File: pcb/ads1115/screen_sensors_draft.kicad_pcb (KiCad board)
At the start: 2 copper layers, 42 x 32 mm, 16 parts, among them J1 WAVESHARE_I2C, J2 BOILER_PROBE, J3 XDB401_ANALOG, U1 ADS1115IDGSR, U2 SHT40-AD1B

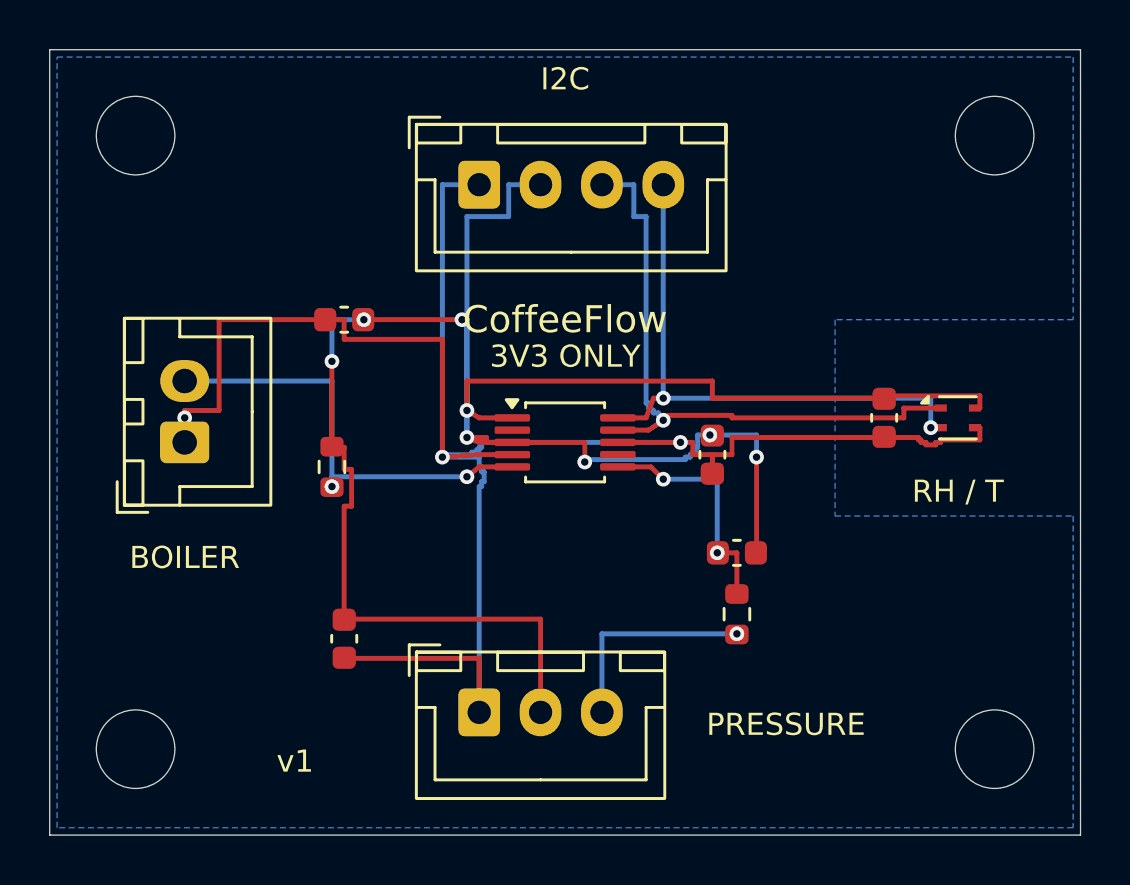
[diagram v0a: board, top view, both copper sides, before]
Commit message: pcb manual rework
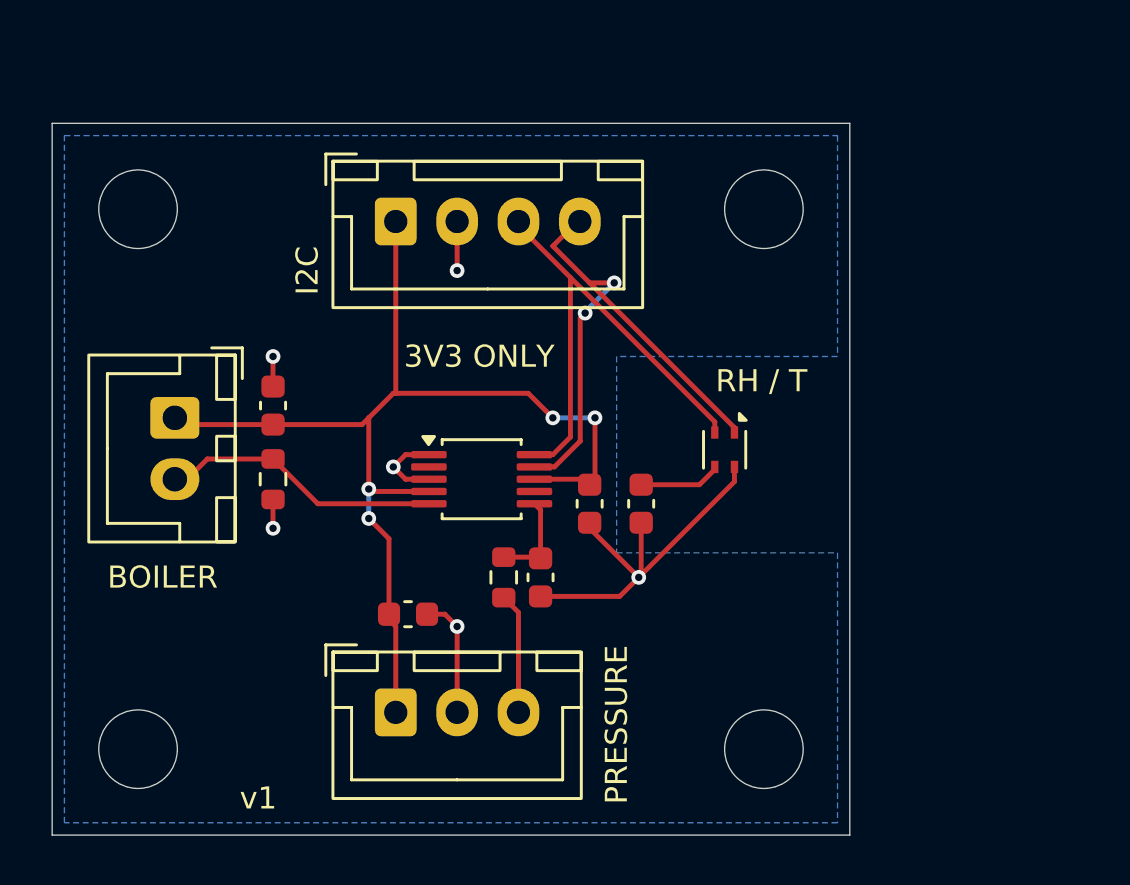
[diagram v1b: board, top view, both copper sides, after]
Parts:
- moved C6 10.5 mm to (124.1, 118.5), turned to -90 degrees
- moved H2 9.87 mm to (129.1, 106.5)
- moved R3 9.62 mm to (118.5, 121.5)
- moved U2 9.59 mm to (127.5, 116.3), turned to -90 degrees
- moved H4 9.40 mm to (129.1, 128.5)
- moved C4 8.06 mm to (120.0, 121.5), turned to -90 degrees
- moved C1 5.39 mm to (122.0, 118.5), turned to -90 degrees
- moved C2 4.55 mm to (109.1, 114.5), turned to 90 degrees
- moved J1 3.72 mm to (114.1, 107.0)
- moved U1 3.72 mm to (117.6, 117.5)
- moved J3 3.40 mm to (114.1, 127.0)
- moved H1 3.00 mm to (103.6, 106.5)
- moved C5 2.79 mm to (114.6, 123.0), turned to 0 degrees
- moved R1 2.45 mm to (109.1, 117.5), turned to -90 degrees
- moved J2 1.08 mm to (105.1, 115.0), turned to -90 degrees
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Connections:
- J1 pad 3: /SDA -> /SCL
- J1 pad 4: /SCL -> /SDA
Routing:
- net /GND: track 95.3 -> 28.5 mm, vias 8 -> 6
- net /3V3: track 85.8 -> 49.3 mm, vias 3 -> 4
- net /BOILER_ADC: track 18.2 -> 11.4 mm, vias 2 -> 0
- net /PRESS_ADC: track 9.83 -> 3.85 mm, vias 2 -> 0
- net /PRESS_SIGNAL: track 8.73 -> 4.92 mm, vias 1 -> 0
- net /SCL: track 23.6 -> 20.2 mm, vias 2 -> 0
- net /SDA: track 26.1 -> 23.4 mm, vias 1 -> 2
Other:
- board size 42 x 32 mm -> 32.5 x 29 mm
- board text removed: "CoffeeFlow"
